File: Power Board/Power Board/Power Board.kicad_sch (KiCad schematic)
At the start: 15 parts, among them J1 MINIFIT-2-VERT, J10 MINIFIT-2-VERT, J2 MINIFIT-2-VERT, J3 MINIFIT-2-VERT, J4 MEGAFIT-2-VERT, J5 MINIFIT-2-VERT, J6 MINIFIT-2-VERT, J7 MINIFIT-2-VERT, J8 MINIFIT-2-VERT, J9 MINIFIT-2-VERT

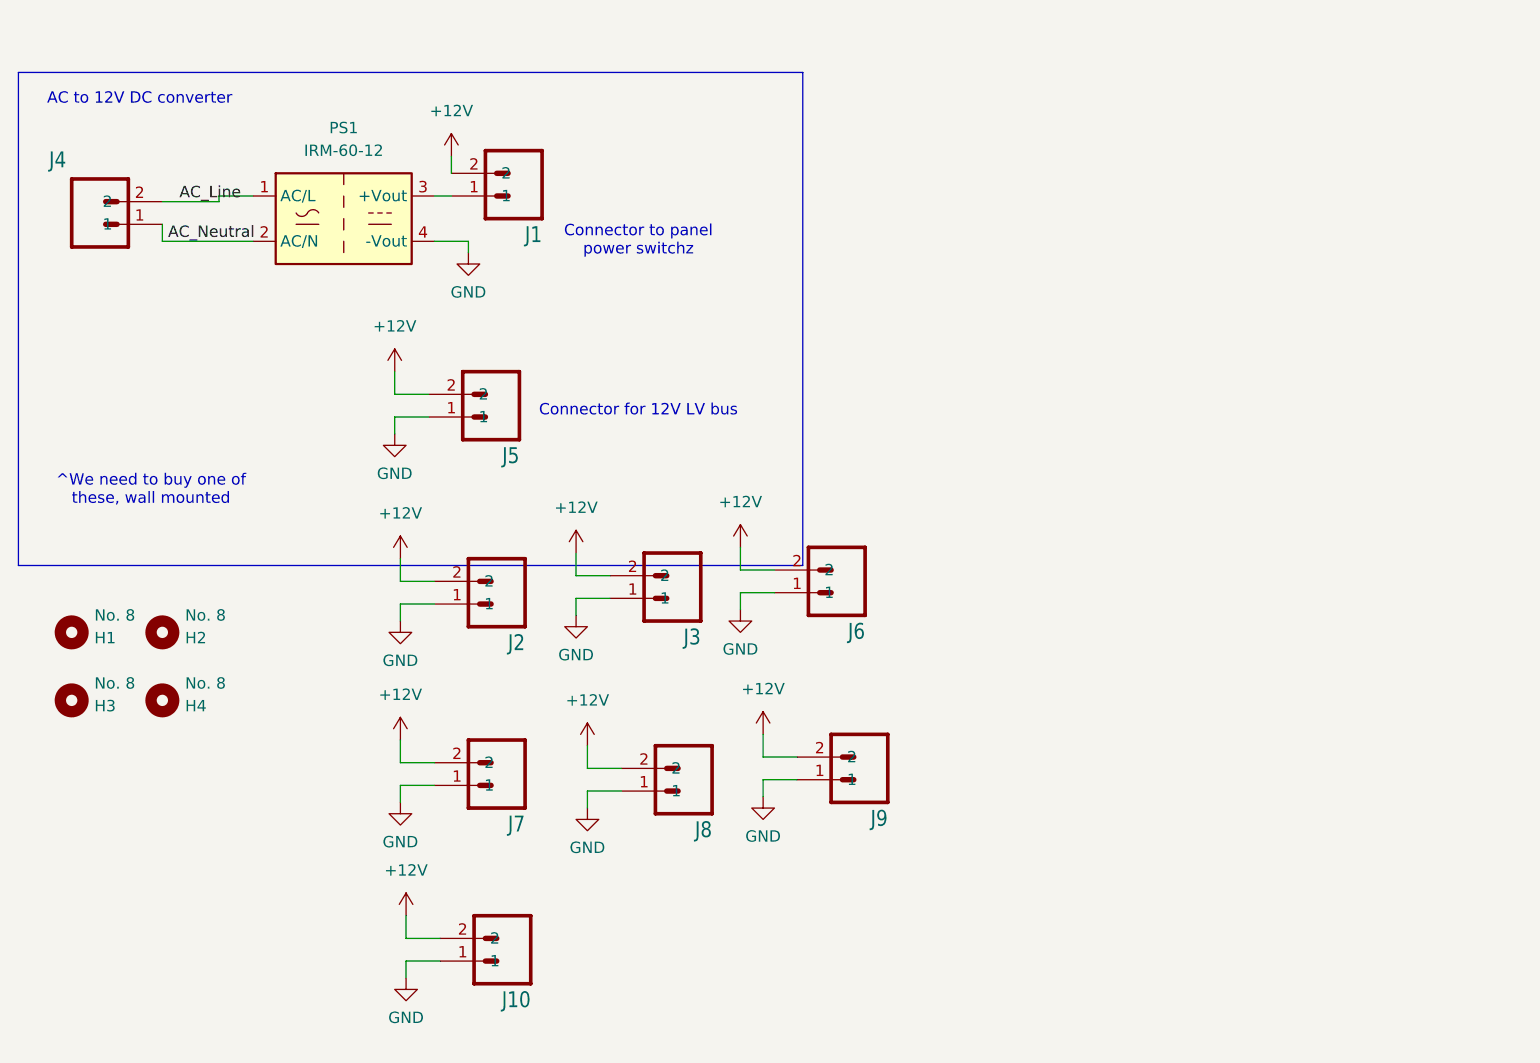
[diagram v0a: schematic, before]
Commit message: Completed Power Board
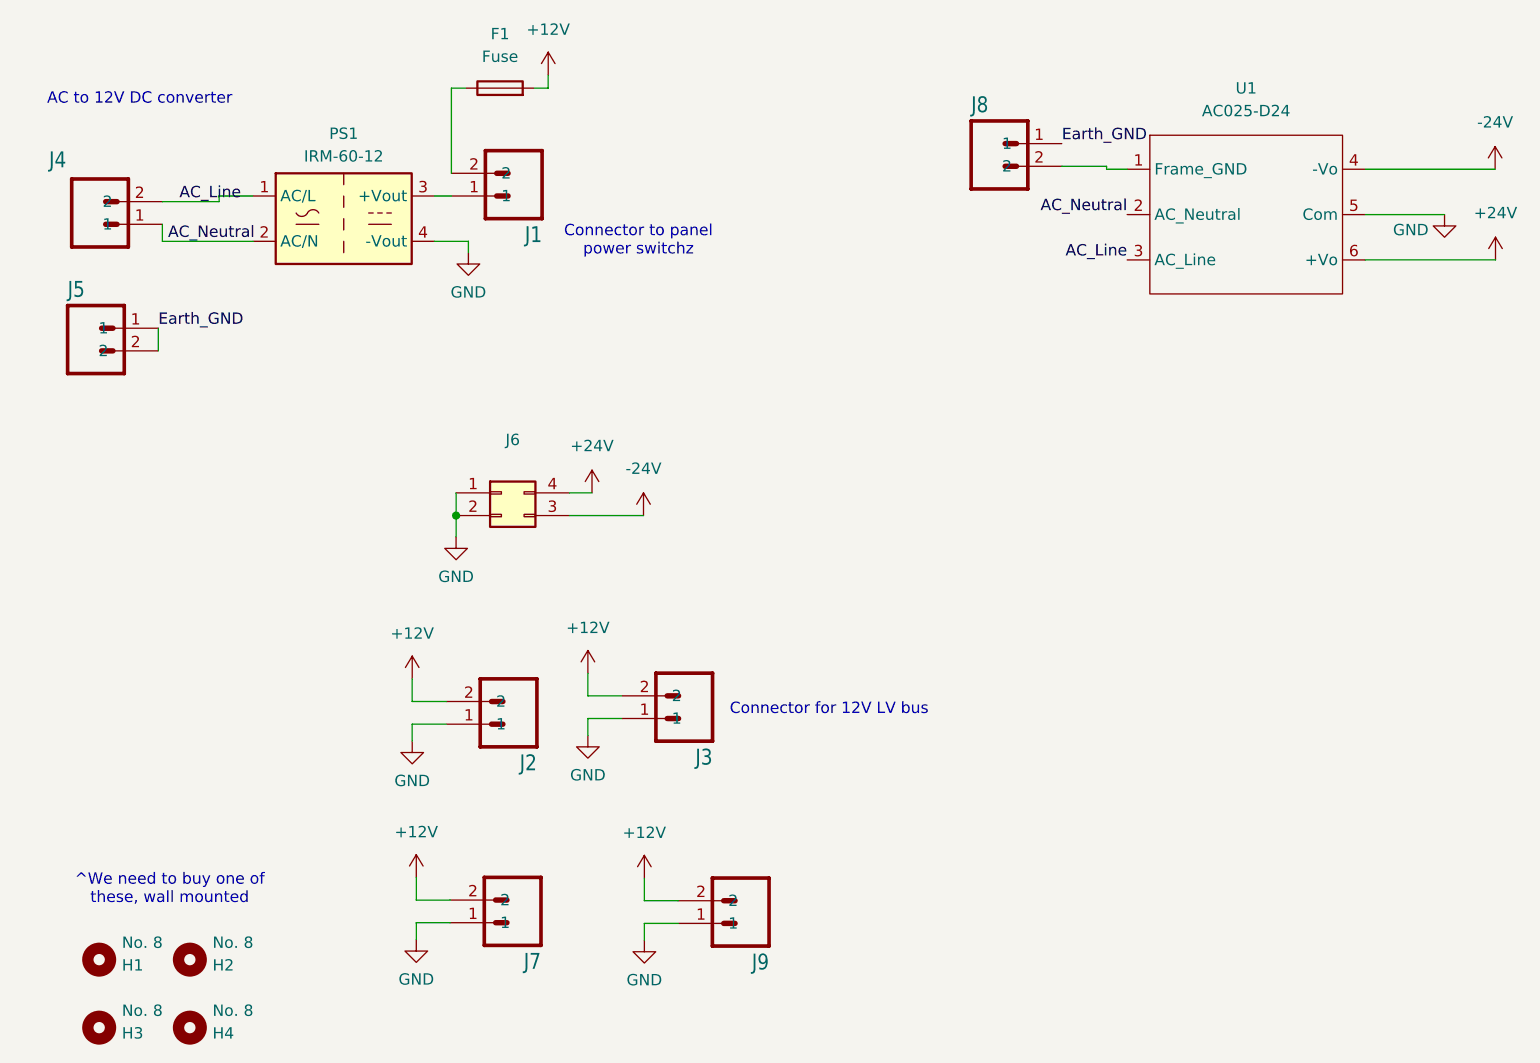
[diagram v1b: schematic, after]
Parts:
- removed J10, J6: MINIFIT-2-VERT, Connector_Molex:Molex_Mini-Fit_Jr_5566-02A_2x01_P4.20mm_Vertical, symbol BMS-Master-Revision8-eagle-import:MINIFIT-2-VERT
- added F1: Fuse, Fuse:Fuseholder_Blade_Mini_Keystone_3568, symbol Device:Fuse
- added J6: ~, Connector_Molex:Molex_Mega-Fit_76829-0004_2x02_P5.70mm_Vertical, symbol Connector_Generic:Conn_02x02_Counter_Clockwise
- added U1: AC025-D24, GTSR_KiCAD_Footprints:AC025-D15, symbol GTSR_symbol_lib:AC025-D15
- J5: footprint Connector_Molex:Molex_Mini-Fit_Jr_5566-02A_2x01_P4.20mm_Vertical -> Connector_Molex:Molex_Micro-Fit_3.0_43650-0215_1x02_P3.00mm_Vertical
- J8: footprint Connector_Molex:Molex_Mini-Fit_Jr_5566-02A_2x01_P4.20mm_Vertical -> Connector_PinHeader_2.54mm:PinHeader_1x02_P2.54mm_Vertical
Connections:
- net +12V: now also F1.2; no longer J1.2, J5.2, J8.2
- net AC_Line: now also U1.3 (AC_Line)
- net AC_Neutral: now also U1.2 (AC_Neutral)
- net GND: now also J6.1 (Pin_1), J6.2 (Pin_2), U1.5 (Com); no longer J5.1, J8.1
- new net: J8.2, U1.1 (Frame_GND)
- new net: F1.1, J1.2
- new net +24V: J6.4 (Pin_4), U1.6 (+Vo)
- new net -24V: J6.3 (Pin_3), U1.4 (-Vo)
- new net Earth_GND: J5.1, J5.2, J8.1
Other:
- moved on the sheet: H1, H2, H3, H4, J2, J3
